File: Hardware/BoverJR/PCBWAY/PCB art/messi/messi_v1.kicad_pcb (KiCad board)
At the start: 2 copper layers, 35 x 35 mm, 4 parts

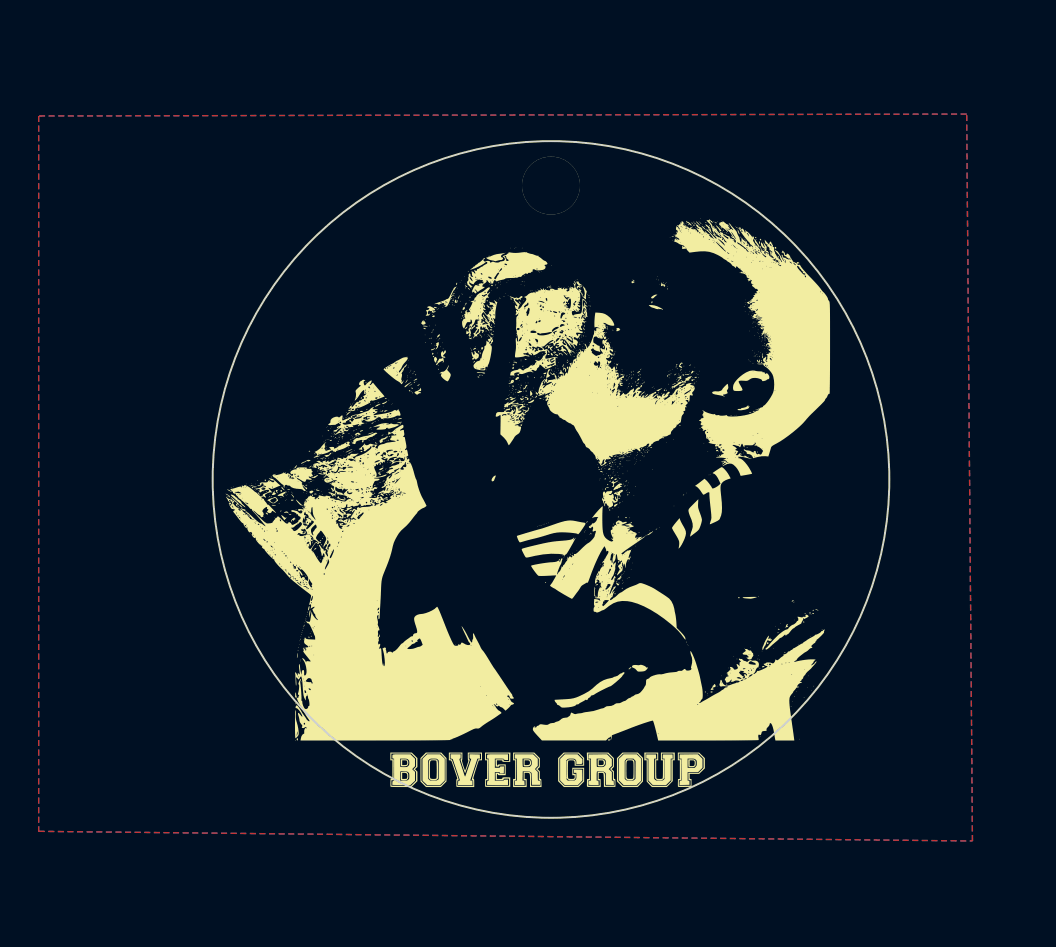
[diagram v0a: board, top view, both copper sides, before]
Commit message: terrmine llavero messi
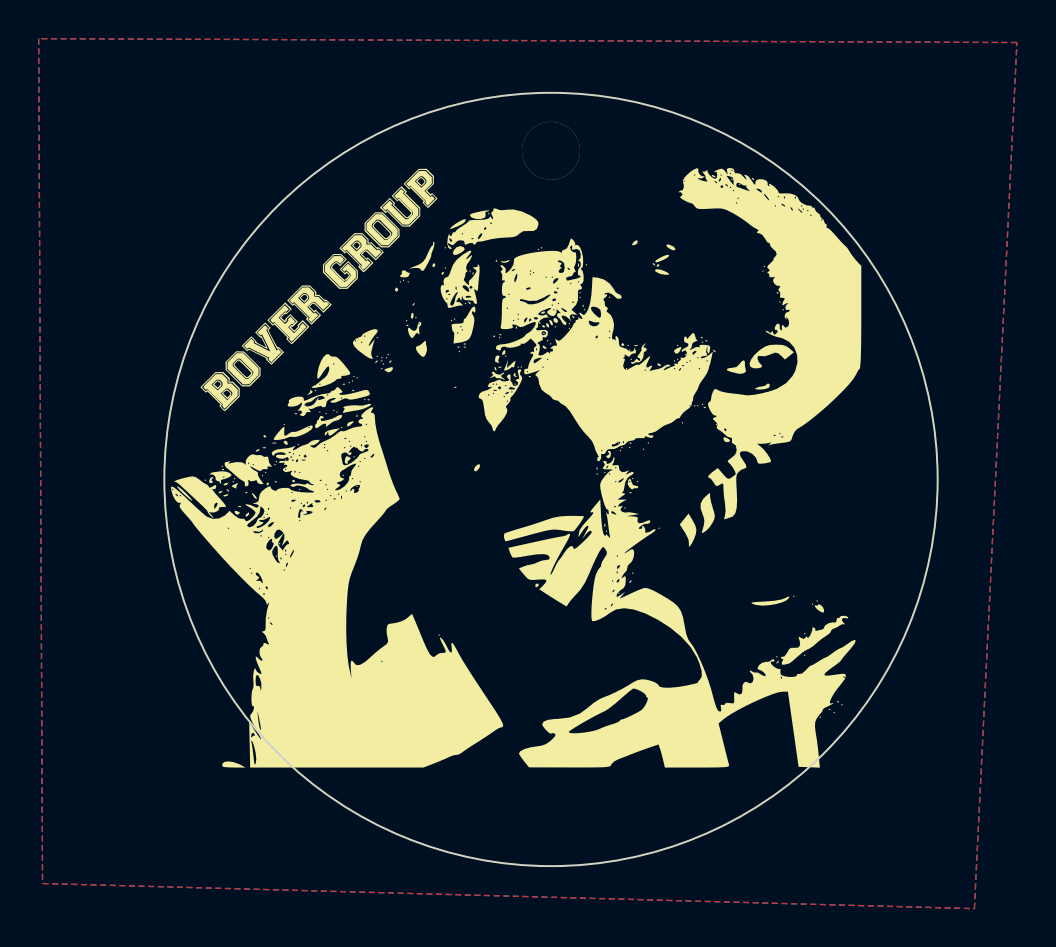
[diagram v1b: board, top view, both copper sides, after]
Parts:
- added H5: Mounting_Hole, EESTN5:afa_mm, F.Cu at (126.2, 91.8)
- added H6: Mounting_Hole, EESTN5:bover_mm, F.Cu at (153.2, 93.4)
- H2: footprint EESTN5:logo_messiv3 -> EESTN5:messi
- moved H3 27.6 mm to (128.4, 86.2), turned to 45 degrees
- moved H1 1.80 mm to (140.0, 79.2)
- moved H2 1.43 mm to (136.0, 91.1)
- moved H4 0.36 mm to (139.6, 97.8)
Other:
- board size 35 x 35 mm -> 40 x 40 mm
